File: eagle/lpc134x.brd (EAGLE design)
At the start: 39.8 x 24.7 mm, 37 parts, among them IC2 LT1763CS8-3.3, Q1 12Mhz, SW1 SWITCH_MCTAEF, T1 Si2301DS, X1 USB-MICROB

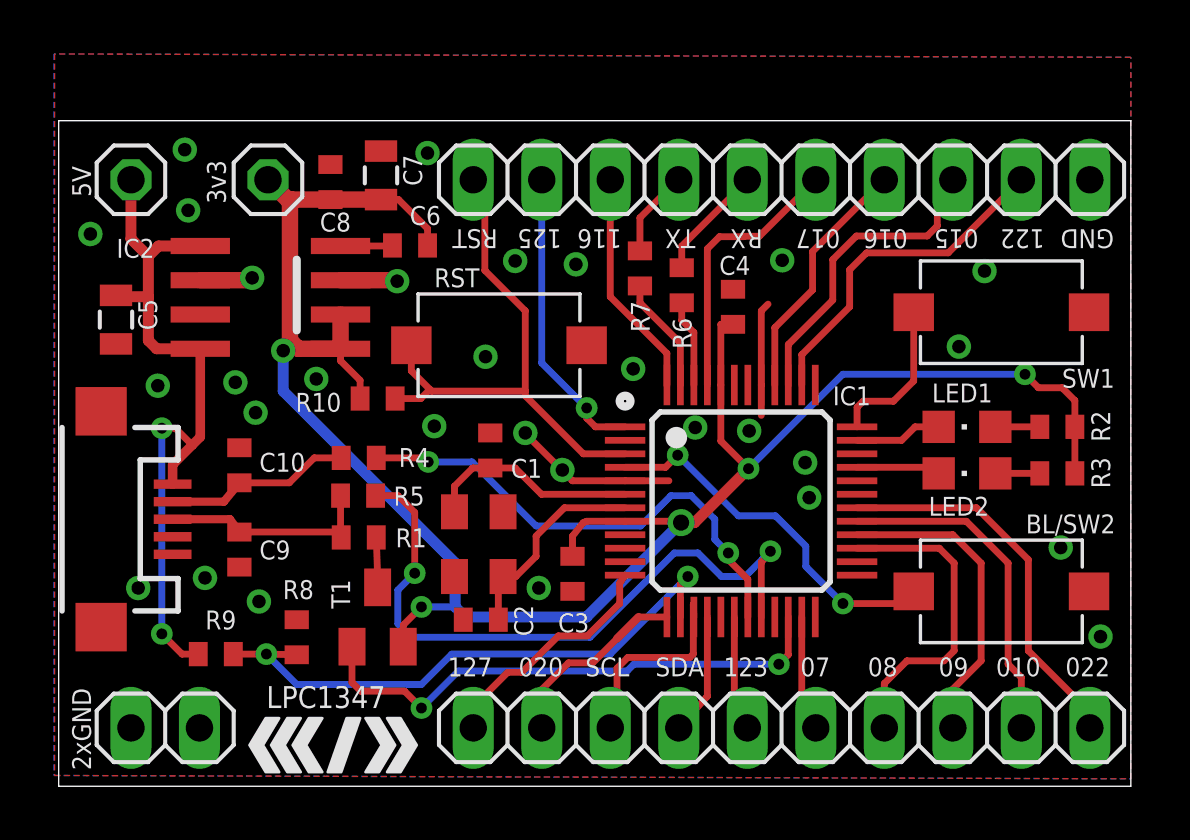
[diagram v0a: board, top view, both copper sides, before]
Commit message: pcb update
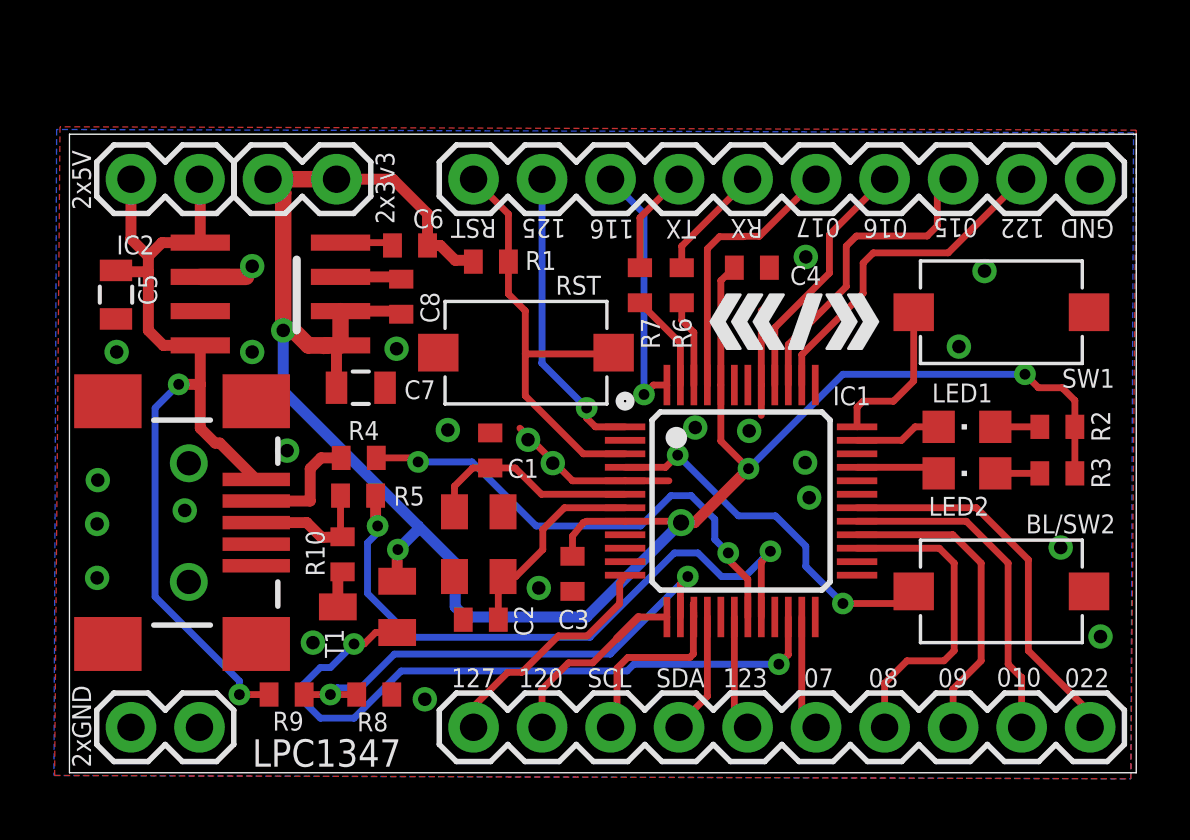
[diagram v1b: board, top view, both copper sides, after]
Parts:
- removed C10, C9: 22pF, rcl:C0402
- removed JP5: (no value), pinhead:1X01
- removed U$1: (no value), seb:C3D2_LOGO
- removed X1: USB-MICROB, SparkFun-Connectors:USB-MICROB
- added JP3: (no value), SparkFun-Connectors:1X02
- added X2: USB-SMD-NS, SparkFun-Connectors:USB-MINIB-NOSTOP
- JP1: value (none) -> M10"; device pinhead-2:1X10 -> SparkFun-Connectors:1X10
- JP2: device pinhead-2:1X10 -> SparkFun-Connectors:1X02
- JP4: device pinhead-2:1X02 -> SparkFun-Connectors:1X02
- JP6: value (none) -> M10"; device pinhead:1X01 -> SparkFun-Connectors:1X10
- R1: value 1k5 -> 15k
- R10: value 15k -> 1k5
- moved JP6 40.9 mm to (37.5, 2.29), turned to 180 degrees
- moved JP2 31.5 mm to (1.98, 2.29)
- moved JP1 23.3 mm to (37.5, 22.6)
- moved U$2 23.2 mm to (23.5, 17.3)
- moved JP4 20.4 mm to (1.98, 22.6)
- moved R1 11.3 mm to (15.3, 19.6), turned to 180 degrees
- moved C7 7.91 mm to (10.5, 14.9), turned to 0 degrees
- moved R10 5.92 mm to (9.82, 8.70), turned to 270 degrees
- moved C8 5.00 mm to (12.0, 18.2)
- moved R8 3.58 mm to (11.0, 3.50), turned to 180 degrees
- moved R9 3.02 mm to (7.75, 3.50)
- moved C4 1.61 mm to (25.0, 19.3), turned to 180 degrees
- moved RST 1.04 mm to (16.6, 16.2), turned to 0 degrees
- moved C5 0.93 mm to (1.43, 18.3)
- moved R7 0.62 mm to (20.9, 18.7)
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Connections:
- net N$14 renamed USB_D-
- net N$24 renamed USB_D+
- net N$3 renamed XTAL_OUT
- net N$4 renamed XTAL_IN
- net +3V3: now also JP3.1, JP3.2, R1.2; no longer JP5.1, R10.2
- net +5V: now also JP4.1, JP4.2, X2.VBUS; no longer JP6.1, X1.VBUS
- net 010: now also JP6.2; no longer JP1.2
- net 015: now also JP1.3; no longer JP2.8
- net 016: now also JP1.4; no longer JP2.7
- net 017: now also JP1.5; no longer JP2.6
- net 022: now also JP6.1; no longer JP1.1
- net 07: now also JP6.5; no longer JP1.5
- net 08: now also JP6.4; no longer JP1.4
- net 09: now also JP6.3; no longer JP1.3
- net 116: now also JP1.8; no longer JP2.3
- net 120: now also JP6.9; no longer JP1.9
- net 122: now also JP1.2; no longer JP2.9
- net 123: now also JP6.6; no longer JP1.6
- net 125: now also JP1.9; no longer JP2.2
- net 127: now also JP6.10; no longer JP1.10
- net GND: now also JP1.1, JP2.1, JP2.2, X2.GND; no longer C10.1, C9.2, JP2.10, JP4.1, JP4.2, X1.GND, X1.MT1, X1.MT2
- net N$10: now also R10.1, X2.D+; no longer C9.1, R1.1, X1.D+
- net N$11: now also X2.D-; no longer C10.2, X1.D-
- net N$20: now also R10.2; no longer R1.2
- net RST: now also JP1.10, R1.1; no longer JP2.1, R10.1
- net RX: now also JP1.6; no longer JP2.5
- net SCL: now also JP6.8; no longer JP1.8
- net SDA: now also JP6.7; no longer JP1.7
- net TX: now also JP1.7; no longer JP2.4
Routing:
- net +5V: track 27.8 -> 34.8 mm
- net +3V3: track 75.2 -> 81.9 mm
- net 06: track 20.1 -> 25.7 mm
- net RST: track 20.3 -> 16.7 mm
- net VBUS: track 21.7 -> 18.6 mm
- net N$10: track 8.33 -> 5.24 mm
- net N$11: track 6.96 -> 4.52 mm
- net 116: track 8.48 -> 9.49 mm, vias 0 -> 1
- net USB_D+: track 25.2 -> 24.5 mm
- net TX: track 3.24 -> 3.89 mm
- net 019: track 4.30 -> 3.67 mm
- net GND: track 14.4 -> 14.5 mm, vias 30 -> 24
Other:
- board size 39.8 x 24.7 mm -> 39.5 x 23.7 mm
- board text added: "120"
- board text added: "2x3v3"
- board text added: "2x5V"
- board text removed: "020"
